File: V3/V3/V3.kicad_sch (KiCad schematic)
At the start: 65 parts, among them J1 Conn_01x04_Pin, J2 Conn_01x04_Pin, J3 Conn_01x06_Pin, J4 Conn_01x07_Pin, J5 2337019-1, Q1 DMP3099L-7, Q2 NMOS, Q3 NMOS, SW1 PTS636 SM50J SMTR LFS, SW2 PTS636 SM50J SMTR LFS, U1 W25Q16JVSSIQ, U2 MAX-M10M-00B, U3 ESP32-WROOM-32UE, U4 BMI088, U5 MMC5983MA, U6 MS560702BA03-50

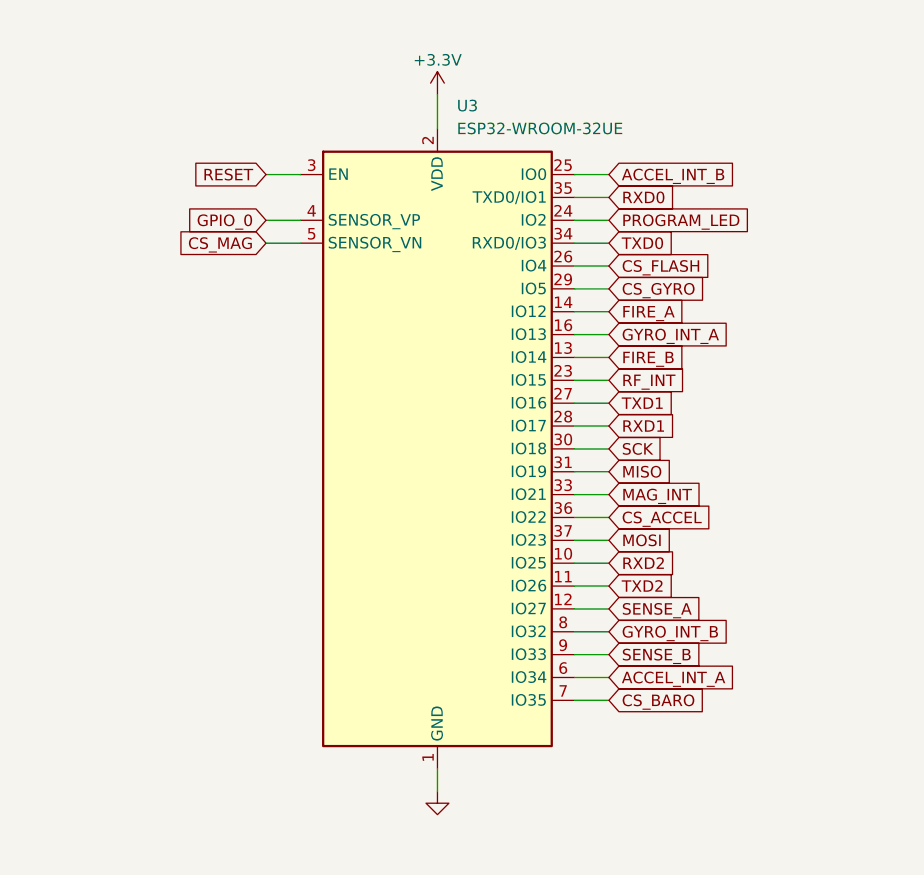
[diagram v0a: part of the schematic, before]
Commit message: V3 changes
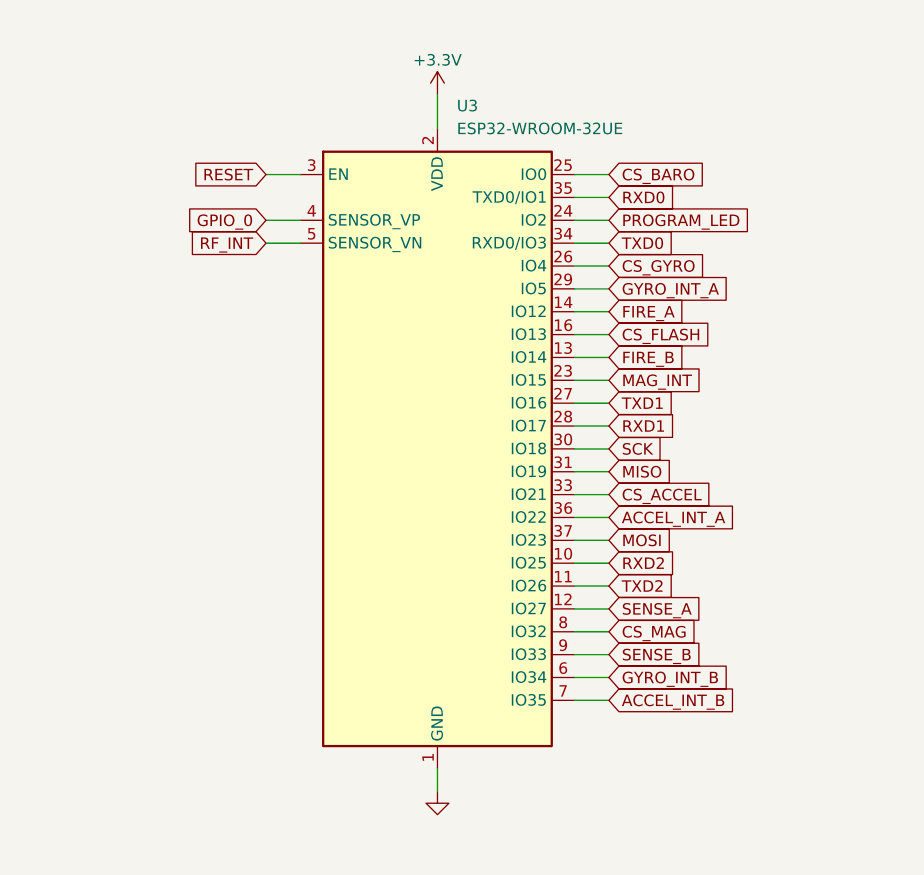
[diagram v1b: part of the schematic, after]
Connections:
- net ACCEL_INT_A: now also U3.36 (IO22); no longer U3.6 (IO34)
- net ACCEL_INT_B: now also U3.7 (IO35); no longer U3.25 (IO0)
- net CS_ACCEL: now also U3.33 (IO21); no longer U3.36 (IO22)
- net CS_BARO: now also U3.25 (IO0); no longer U3.7 (IO35)
- net CS_FLASH: now also U3.16 (IO13); no longer U3.26 (IO4)
- net CS_GYRO: now also U3.26 (IO4); no longer U3.29 (IO5)
- net CS_MAG: now also U3.8 (IO32); no longer U3.5 (SENSOR_VN)
- net GYRO_INT_A: now also U3.29 (IO5); no longer U3.16 (IO13)
- net GYRO_INT_B: now also U3.6 (IO34); no longer U3.8 (IO32)
- net MAG_INT: now also U3.23 (IO15); no longer U3.33 (IO21)
- net RF_INT: now also U3.5 (SENSOR_VN); no longer U3.23 (IO15)
